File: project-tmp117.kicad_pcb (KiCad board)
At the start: 2 copper layers, 17 parts, among them J1 Conn_01x01_Pin, J2 Conn_01x01_Pin, J3 Conn_01x01_Pin, J4 Conn_01x01_Pin, J5 Conn_01x01_Pin, J7 SM04B-SRSS-TB(LF)(SN), J8 SM04B-SRSS-TB(LF)(SN), U1 TMP117AIDRVR

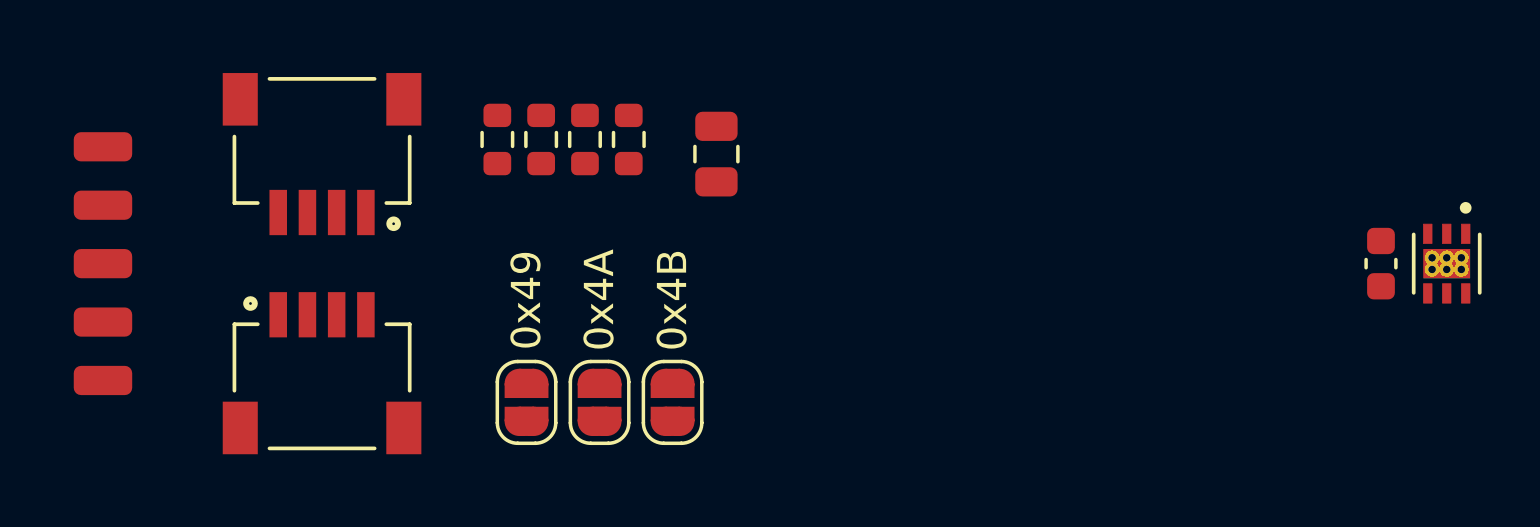
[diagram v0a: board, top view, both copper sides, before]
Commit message: Routing in progress
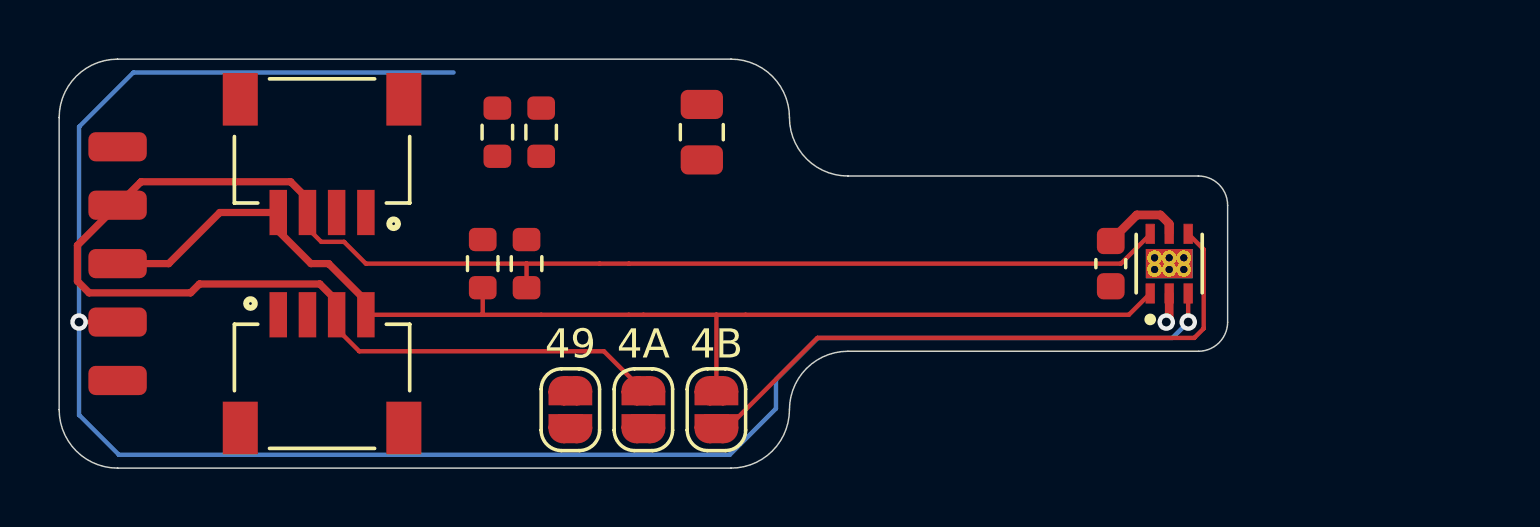
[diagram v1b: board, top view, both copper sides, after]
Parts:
- JP1: value 0x49 -> 49
- JP2: value 0x4A -> 4A
- JP3: value 0x4B -> 4B
- moved U1 9.50 mm to (56.0, 24.2), turned to 90 degrees
- moved C1 9.25 mm to (54.0, 24.2), turned to -90 degrees
- moved R2 5.51 mm to (34.0, 24.2)
- moved R4 5.51 mm to (32.5, 24.2)
- moved J2 2.06 mm to (20.0, 22.2)
- moved J3 2.06 mm to (20.0, 24.2)
- moved JP1 1.52 mm to (35.5, 29.2)
- moved JP2 1.52 mm to (38.0, 29.2)
- moved JP3 1.52 mm to (40.5, 29.2)
- moved C2 0.90 mm to (40.0, 19.8)
- moved J1 0.50 mm to (20.0, 20.2)
- moved J4 0.50 mm to (20.0, 26.2)
- moved J5 0.50 mm to (20.0, 28.2)
- moved R1 0.25 mm to (34.5, 19.8)
- moved R3 0.25 mm to (33.0, 19.8)
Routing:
- net /INT: track 0.00 -> 66.7 mm, vias 0 -> 2
- net /SDA: track 0.00 -> 63.6 mm
- net /SCL: track 0.00 -> 42.0 mm
- net /ADD0: track 0.00 -> 21.6 mm
- net VCC: track 0.00 -> 2.84 mm
- net GND: track 0.00 -> 1.02 mm, vias 0 -> 1
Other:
- board outline added: 40 x 14 mm
